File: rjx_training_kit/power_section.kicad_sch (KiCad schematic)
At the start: 12 parts, among them J1 Barrel_Jack_Switch, J2 USB_B_Mini, SW1 SW_SPDT, U6 MPM3610GQV-P

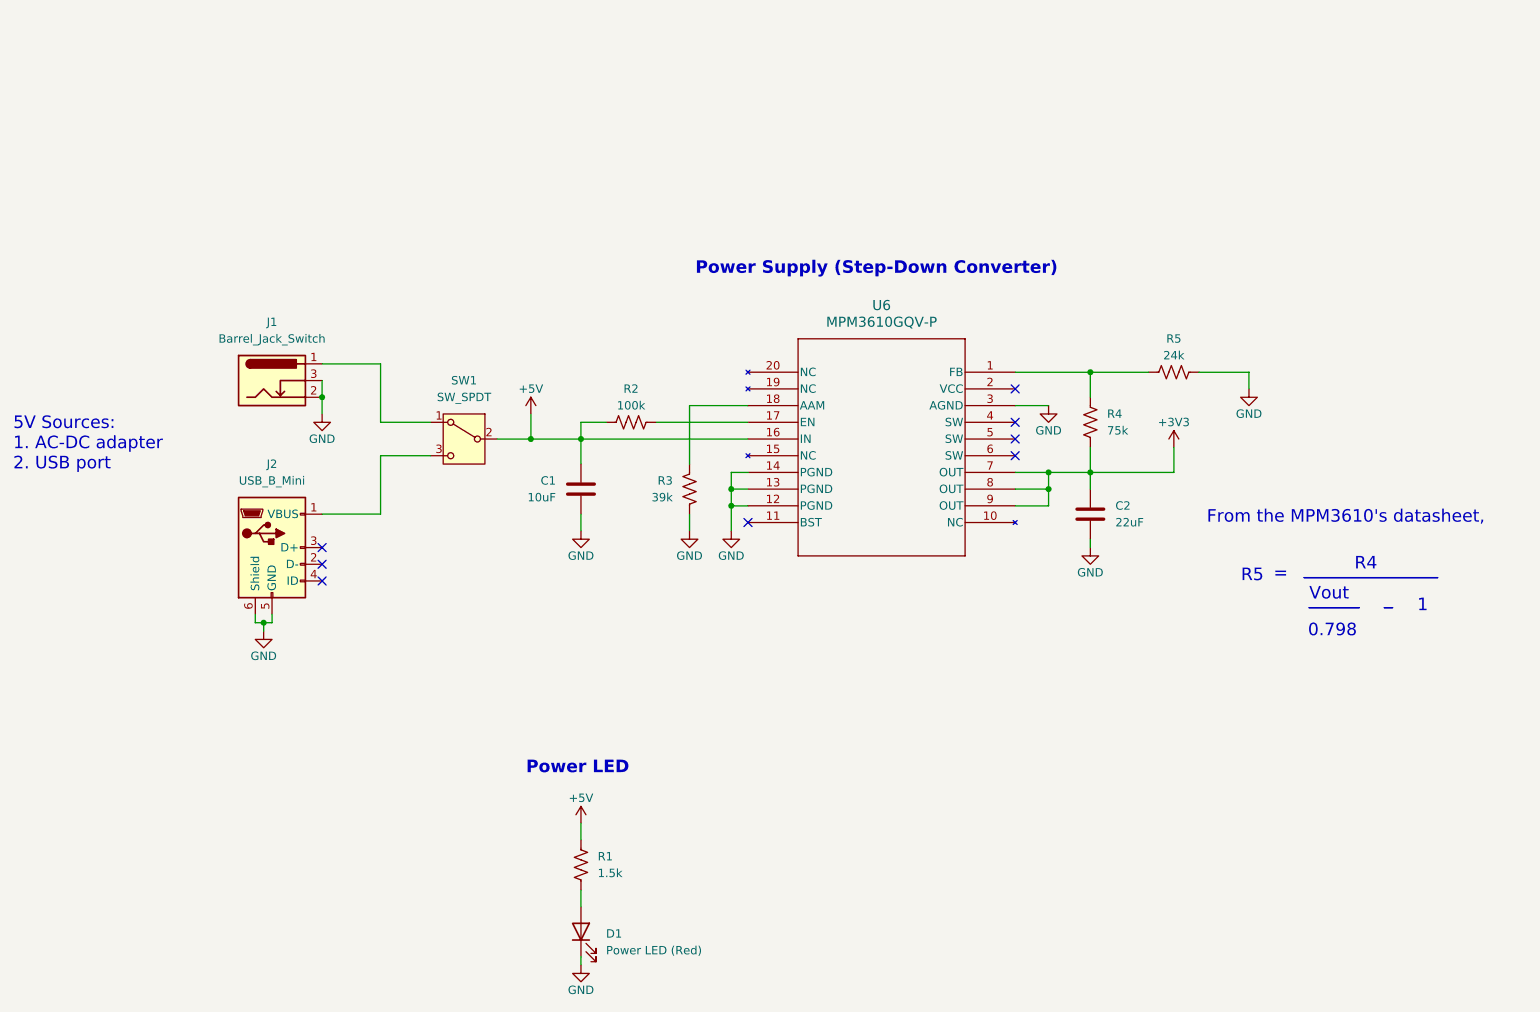
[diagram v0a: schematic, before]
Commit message: Update
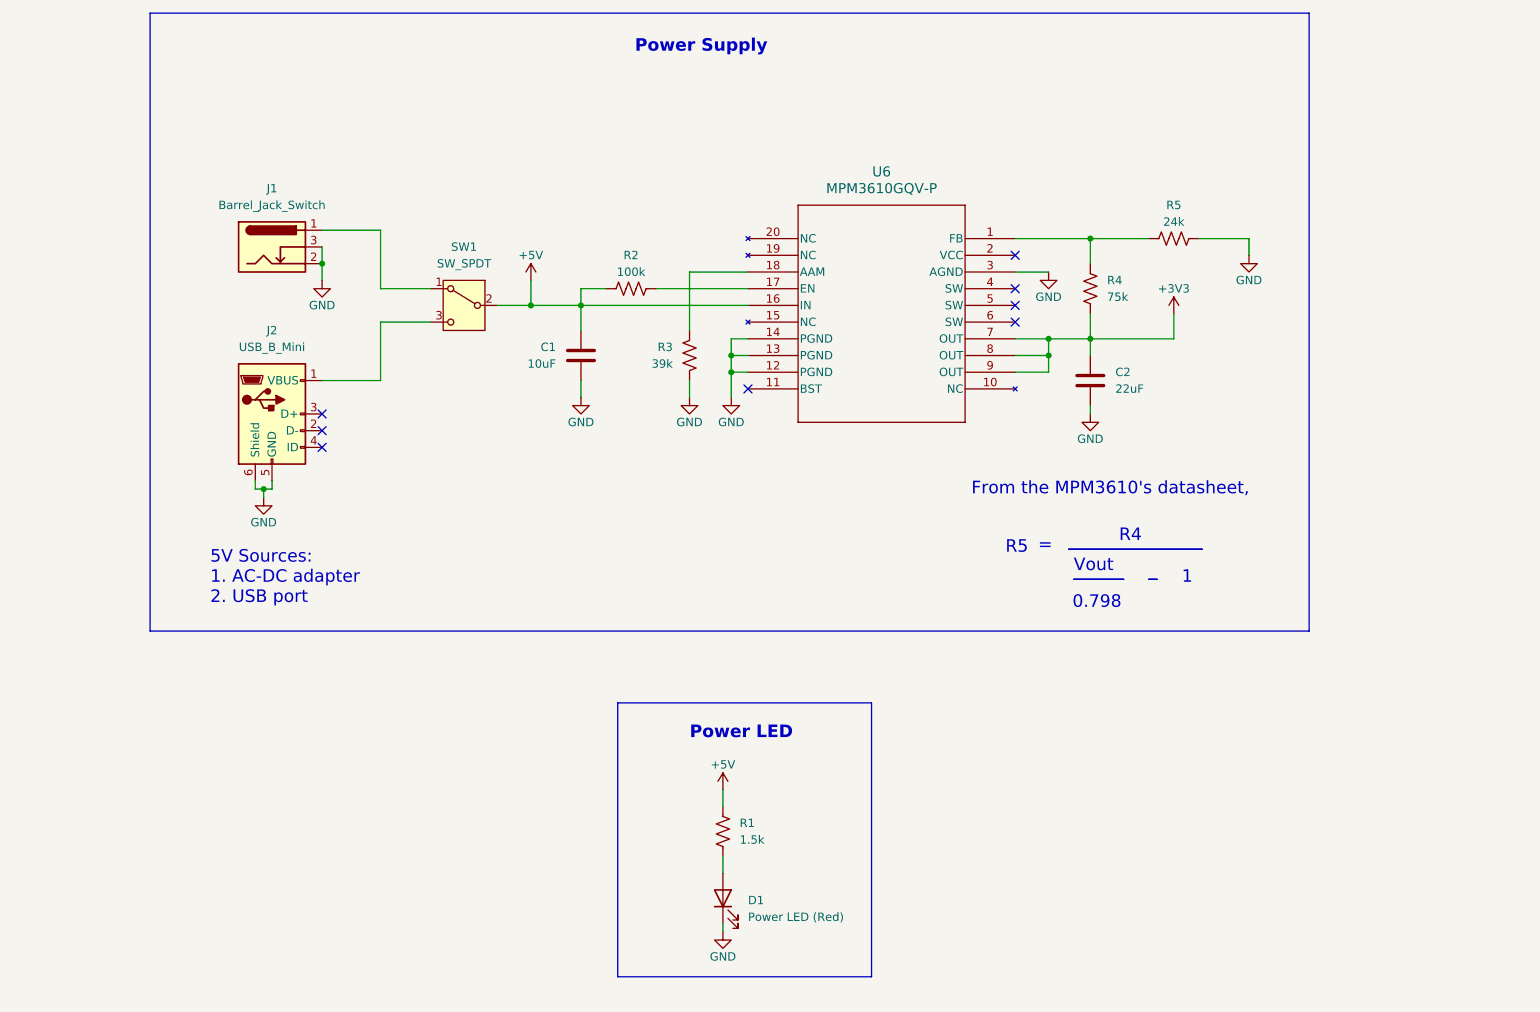
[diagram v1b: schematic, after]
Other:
- note added: "Power Supply"
- note removed: "Power Supply (Step-Down Converter)"
- moved on the sheet: C1, C2, D1, J1, J2, R1, R2, R3, R4, R5, SW1, U6
